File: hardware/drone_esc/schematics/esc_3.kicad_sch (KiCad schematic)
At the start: 32 parts, among them Q13 BSC016N04LS, Q14 BSC016N04LS, Q15 BSC016N04LS, Q16 BSC016N04LS, Q17 BSC016N04LS, Q18 BSC016N04LS, U7 FD6288Q

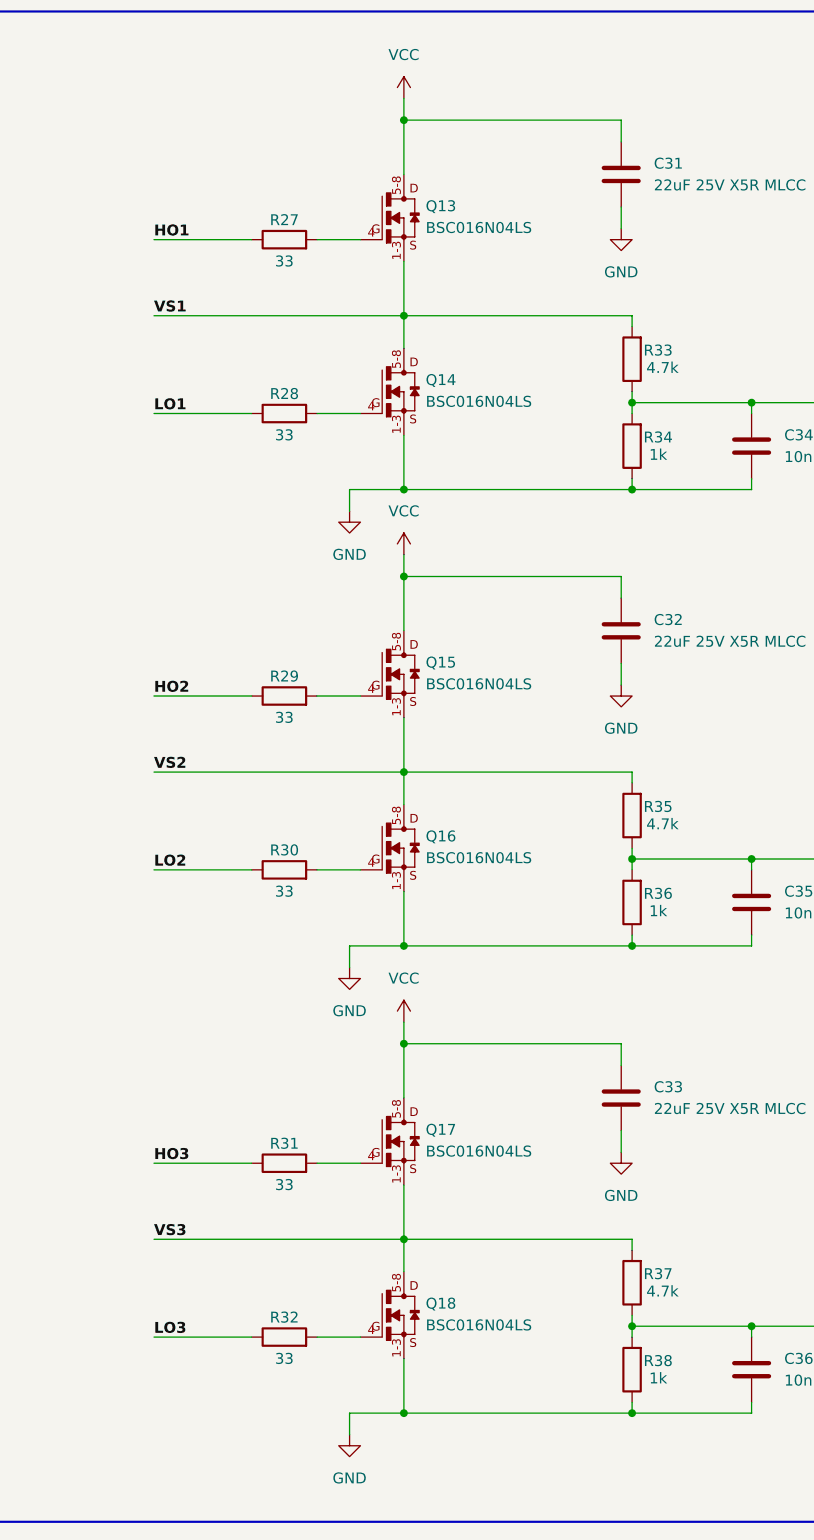
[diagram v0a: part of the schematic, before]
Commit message: replaced some of the schematics
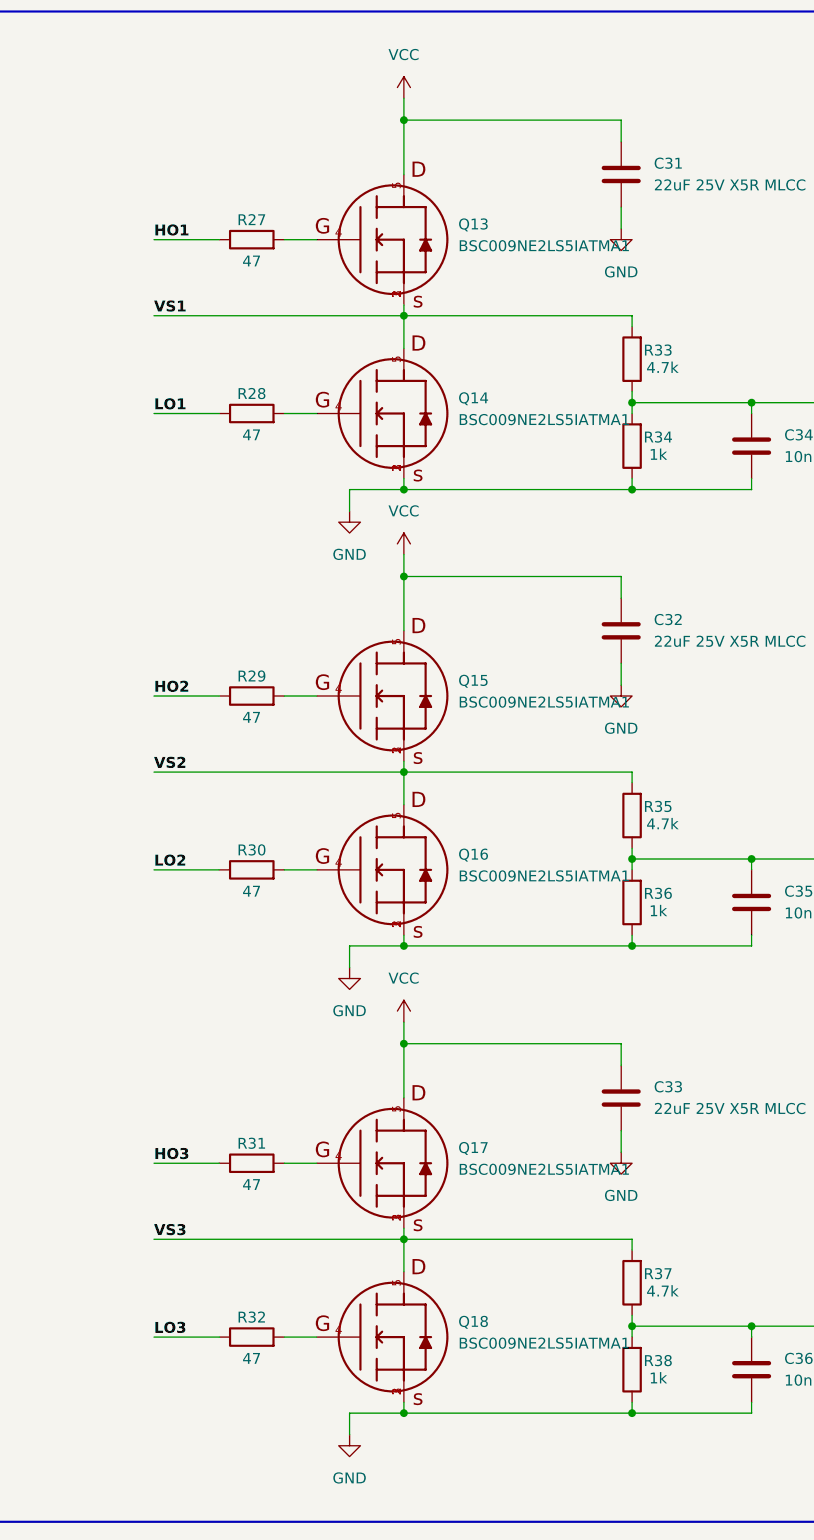
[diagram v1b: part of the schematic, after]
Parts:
- removed Q13, Q14, Q15, Q16, Q17, Q18: BSC016N04LS, Drone_components:BSC016N04LS, symbol Drone_components:BSC016N04LS
- added Q13, Q14, Q15, Q16, Q17, Q18: BSC009NE2LS5IATMA1, Drone_components:BSC093N04LSGATMA1, symbol Drone_components:BSC009NE2LS5IATMA1
- C31, C32, C33: footprint Capacitor_SMD:C_1210_3225Metric -> Capacitor_SMD:C_0805_2012Metric; JLCPCB part C12891 -> C45783
- R27, R28, R29, R30, R31, R32: value 33 -> 47
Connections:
- net GND: now also Q14.1, Q14.2, Q14.3, Q16.1, Q16.2, Q16.3, Q18.1, Q18.2, Q18.3
- net VCC: now also Q13.5, Q15.5, Q17.5
- net VS1: now also Q13.1, Q13.2, Q13.3, Q14.5
- net VS2: now also Q15.1, Q15.2, Q15.3, Q16.5
- net VS3: now also Q17.1, Q17.2, Q17.3, Q18.5
- net at R28.2: now also Q14.4
- net at R32.2: now also Q18.4
- net at R31.2: now also Q17.4
- net at R30.2: now also Q16.4
- net at R27.2: now also Q13.4
- net at R29.2: now also Q15.4
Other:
- moved on the sheet: R27, R28, R29, R30, R31, R32
